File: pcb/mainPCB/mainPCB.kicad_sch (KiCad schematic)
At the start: 4 parts, among them J1 Conn_01x30, J2 Conn_02x15_Counter_Clockwise, U1 ESP32-S3-DevKitC

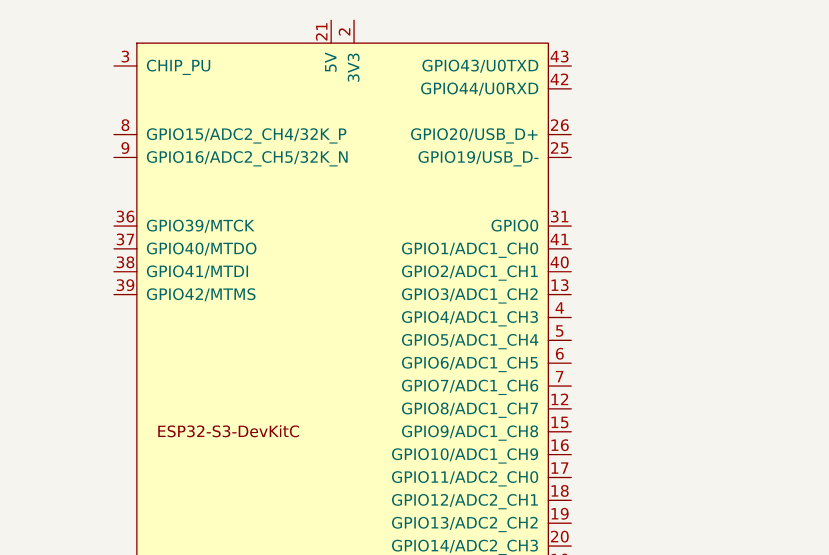
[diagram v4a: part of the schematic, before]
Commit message: wip: starting no crossing cable
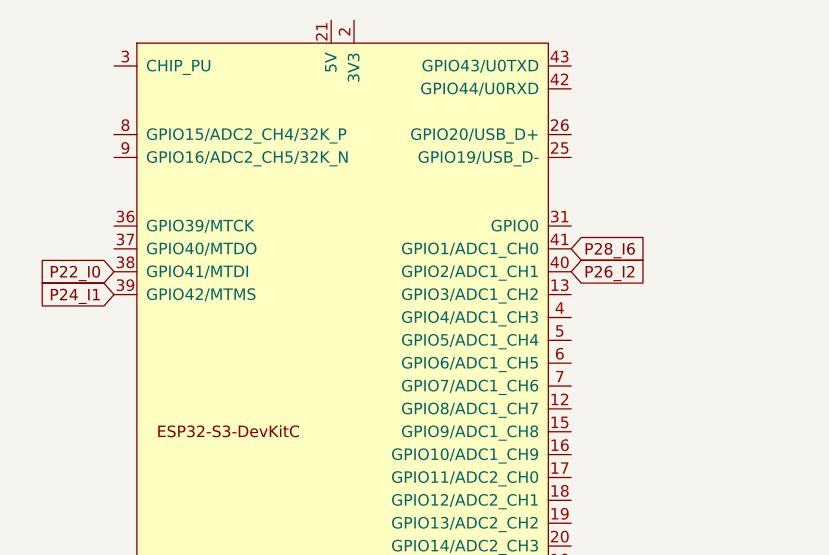
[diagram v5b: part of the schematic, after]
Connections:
- net P22_I0: now also U1.38 (GPIO41/MTDI)
- net P24_I1: now also U1.39 (GPIO42/MTMS)
- net P26_I2: now also U1.40 (GPIO2/ADC1_CH1)
- net P28_I6: now also U1.41 (GPIO1/ADC1_CH0)
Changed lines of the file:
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@@
+		)
+	)
+	(global_label "P28_I6"
+		(shape input)
+		(at 154.94 77.47 0)
+		(fields_autoplaced yes)
+		(effects
+			(font
+				(size 1.27 1.27)
+			)
+			(justify left)
+		)
+		(property "Intersheetrefs" "${INTERSHEET_REFS}"
+			(at 164.3961 77.47 0)
+			(effects
+				(font
+					(size 1.27 1.27)
+				)
+				(justify left)
+				(hide yes)
+			)
 		)
 	)
@@
 		)
 	)
+	(global_label "P26_I2"
+		(shape input)
+		(at 154.94 80.01 0)
+		(fields_autoplaced yes)
+		(effects
+			(font
+				(size 1.27 1.27)
+			)
+			(justify left)
+		)
+		(property "Intersheetrefs" "${INTERSHEET_REFS}"
+			(at 164.3961 80.01 0)
+			(effects
+				(font
+					(size 1.27 1.27)
+				)
+				(justify left)
+				(hide yes)
+			)
+		)
+	)
 	(global_label "P07_O9"
 		(shape input)
@@
 	(global_label "P22_I0"
 		(shape input)
+		(at 104.14 80.01 180)
+		(fields_autoplaced yes)
+		(effects
+			(font
+				(size 1.27 1.27)
+			)
+			(justify right)
+		)
+		(property "Intersheetrefs" "${INTERSHEET_REFS}"
+			(at 94.6839 80.01 0)
+			(effects
+				(font
+					(size 1.27 1.27)
+				)
+				(justify right)
+				(hide yes)
+			)
+		)
+	)
+	(global_label "P22_I0"
+		(shape input)
 		(at 212.09 111.76 180)
 		(fields_autoplaced yes)
@@
 				(hide yes)
 			)
+		)
+	)
+	(global_label "P24_I1"
+		(shape input)
+		(at 104.14 82.55 180)
+		(fields_autoplaced yes)
+		(effects
+			(font
+				(size 1.27 1.27)
+			)
+			(justify right)
+		)
+		(property "Intersheetrefs" "${INTERSHEET_REFS}"
+			(at 94.6839 82.55 0)
+			(effects
+				(font
+					(size 1.27 1.27)
+				)
+				(justify right)
+				(hide yes)
+			)
